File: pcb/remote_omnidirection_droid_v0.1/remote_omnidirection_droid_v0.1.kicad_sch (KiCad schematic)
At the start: 30 parts, among them J1 USB_C_Receptacle_USB2.0, J4 Conn_01x02, Q1 BC846BS, SW1 SW_SPST, U1 USBLC6-2SC6, U3 AZ1117-3.3, U4 AZ1117-5.0, U5 ESP32-S3-WROOM-2-N32R8V

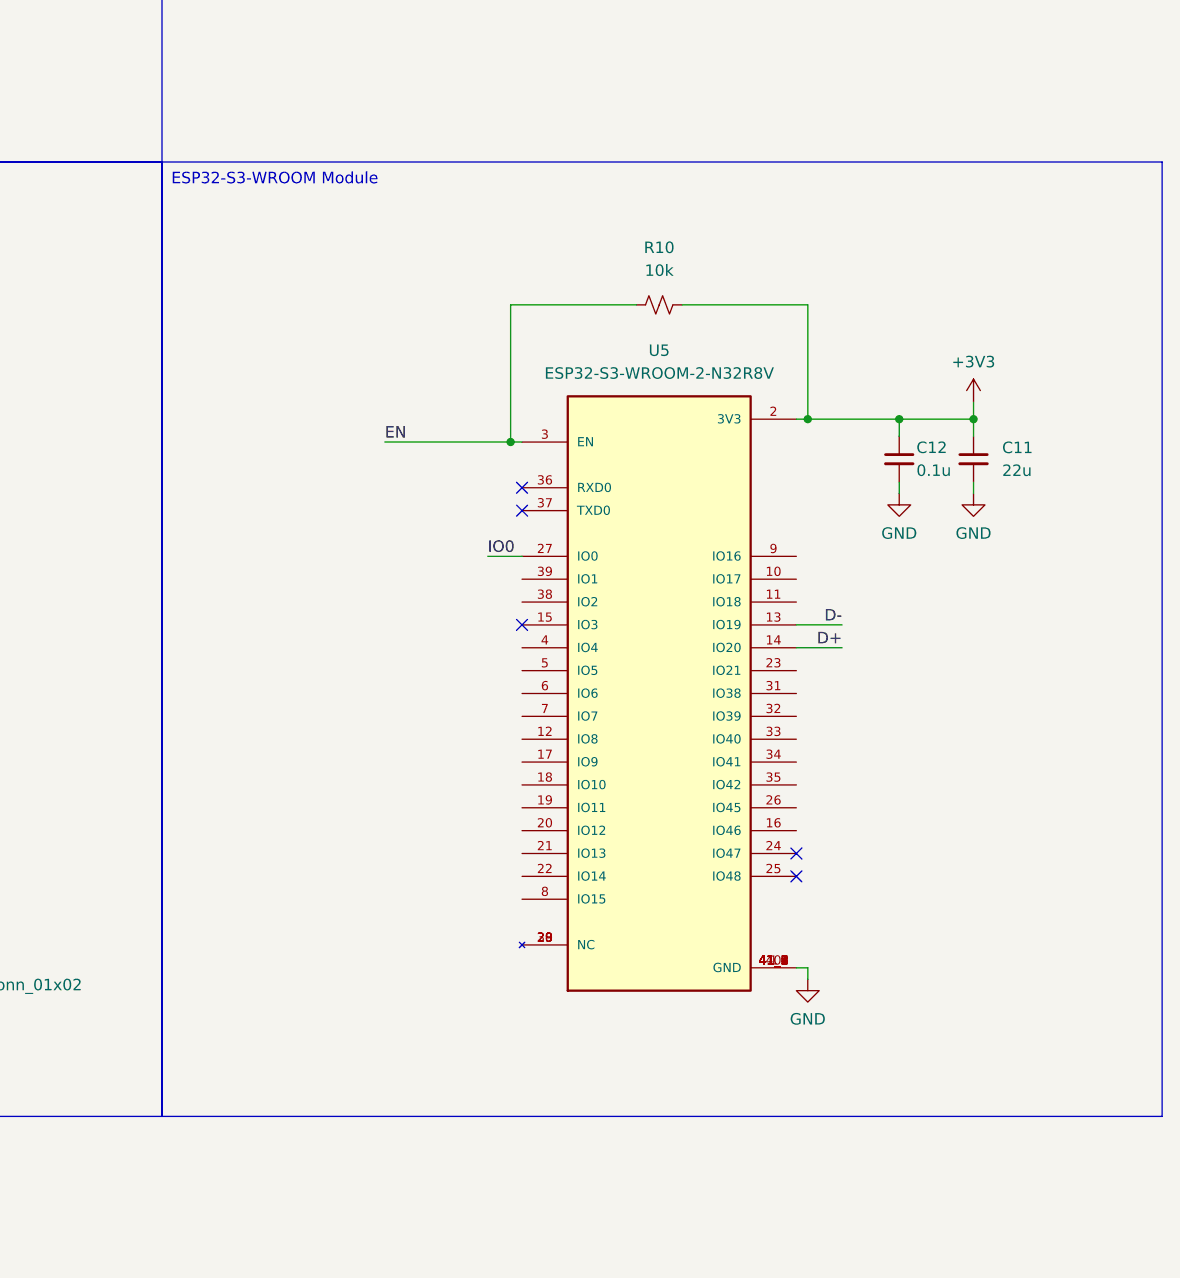
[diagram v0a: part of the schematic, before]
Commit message: poorly designed a PCB
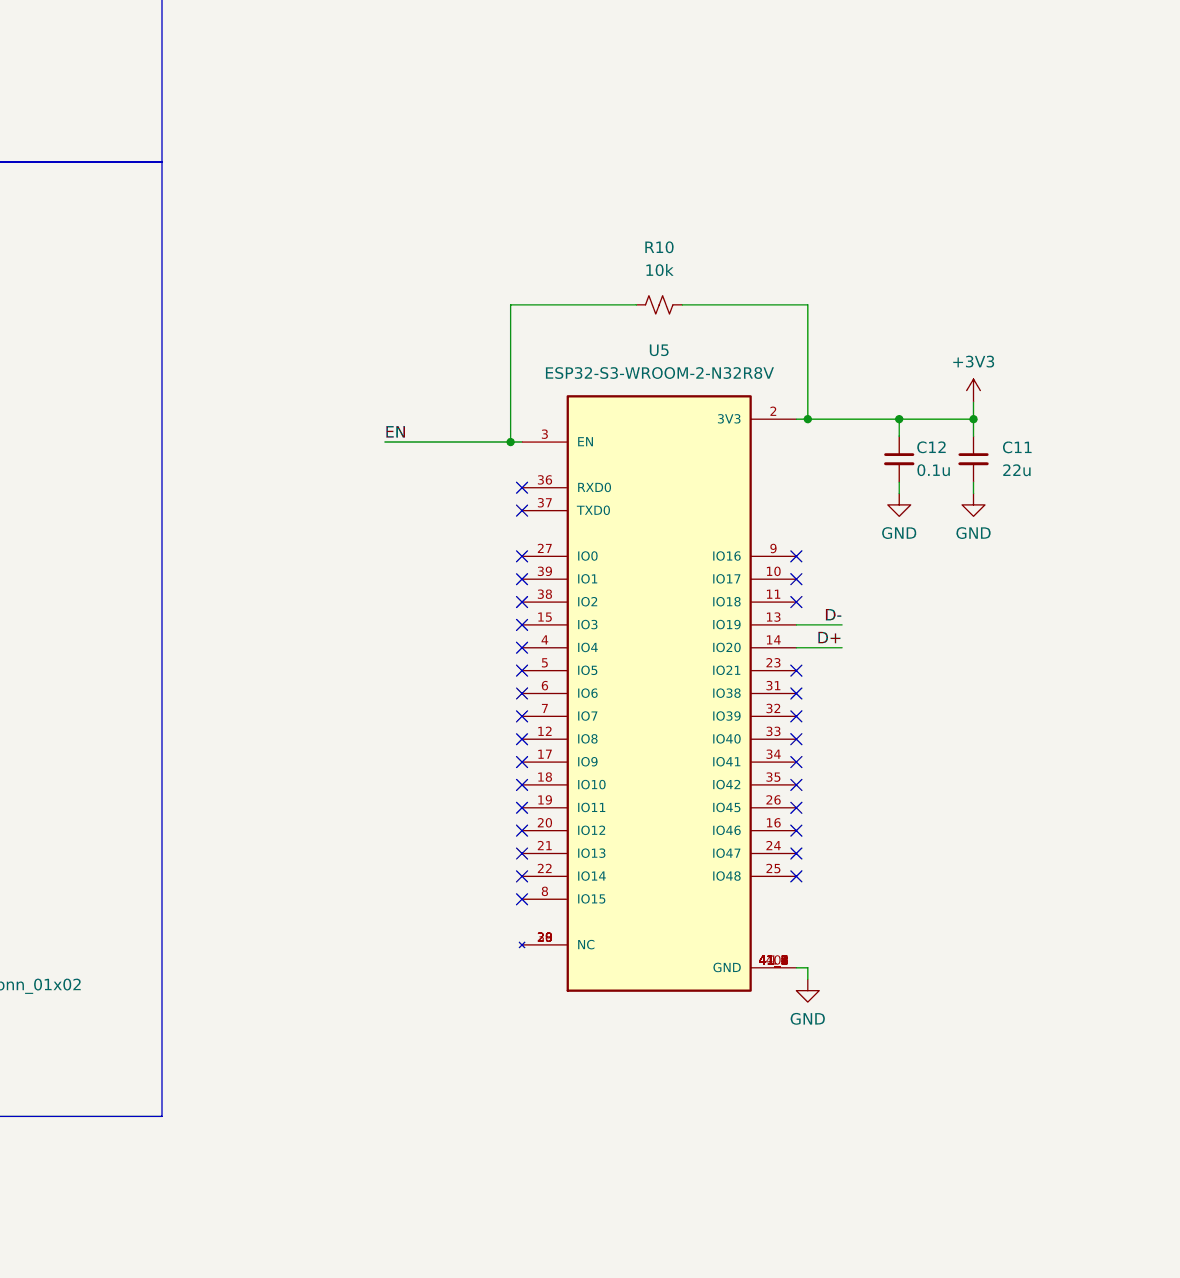
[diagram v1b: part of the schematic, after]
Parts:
- C11, C12, C17: footprint (none) -> Capacitor_SMD:C_1206_3216Metric_Pad1.33x1.80mm_HandSolder
- D1, D2, D8, D9: footprint (none) -> LED_SMD:LED_1206_3216Metric_Pad1.42x1.75mm_HandSolder
- D3, D7: footprint (none) -> Diode_SMD:D_1206_3216Metric_Pad1.42x1.75mm_HandSolder
- J4: footprint (none) -> TestPoint:TestPoint_2Pads_Pitch5.08mm_Drill1.3mm
- R10, R11, R5, R6, R7, R8: footprint (none) -> Resistor_SMD:R_1206_3216Metric_Pad1.30x1.75mm_HandSolder
- U5: footprint ESP32-S3-WROOM-2-N32R8V:XCVR_ESP32-S3-WROOM-2-N32R8V -> ESP32 S3:XCVR_ESP32-S3-WROOM-2-N32R8V
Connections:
- net IO0: no longer names the net of U5.27 (IO0)
- no-connect marks 7 -> 33
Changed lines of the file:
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@@
   (junction (at 56.515 132.715) (diameter 0) (color 0 0 0 0)
   )
+  (no_connect (at 165.1 160.02))
+  (no_connect (at 195.58 167.64))
+  (no_connect (at 195.58 165.1))
+  (no_connect (at 195.58 157.48))
+  (no_connect (at 165.1 162.56))
+  (no_connect (at 165.1 167.64))
   (no_connect (at 165.1 137.16))
+  (no_connect (at 165.1 147.32))
+  (no_connect (at 195.58 162.56))
+  (no_connect (at 165.1 144.78))
+  (no_connect (at 165.1 180.34))
+  (no_connect (at 195.58 142.24))
+  (no_connect (at 165.1 177.8))
+  (no_connect (at 195.58 170.18))
   (no_connect (at 64.135 75.565))
+  (no_connect (at 195.58 147.32))
   (no_connect (at 195.58 175.26))
+  (no_connect (at 165.1 152.4))
+  (no_connect (at 195.58 144.78))
+  (no_connect (at 165.1 170.18))
   (no_connect (at 195.58 177.8))
   (no_connect (at 165.1 134.62))
+  (no_connect (at 165.1 175.26))
+  (no_connect (at 195.58 160.02))
+  (no_connect (at 195.58 154.94))
+  (no_connect (at 165.1 172.72))
   (no_connect (at 165.1 149.86))
+  (no_connect (at 195.58 172.72))
+  (no_connect (at 165.1 154.94))
+  (no_connect (at 165.1 157.48))
   (no_connect (at 64.135 73.025))
+  (no_connect (at 165.1 142.24))
+  (no_connect (at 165.1 165.1))
   (wire (pts (xy 83.185 187.325) (xy 94.615 187.325))
     (stroke (width 0) (type default))
@@
     (stroke (width 0) (type default))
   )
-  (wire (pts (xy 161.29 142.24) (xy 165.1 142.24))
-    (stroke (width 0) (type default))
-  )
   (wire (pts (xy 31.75 215.9) (xy 38.735 215.9))
     (stroke (width 0) (type default))
@@
     (stroke (width 0) (type default))
   )
-  (text_box "ESP32-S3-WROOM Module"
-    (at 125.095 98.425 0) (size 111.125 106.045)
+  (text_box "Enable/Reset Switch"
+    (at 13.335 204.47 0) (size 45.72 27.305)
     (stroke (width 0) (type default))
     (fill (type none))
     (effects (font (size 1.27 1.27)) (justify left top))
   )
-  (text_box "Enable/Reset Switch"
-    (at 13.335 204.47 0) (size 45.72 27.305)
+  (text_box "Power Management"
+    (at 13.335 98.425 0) (size 111.76 106.045)
     (stroke (width 0) (type default))
     (fill (type none))
     (effects (font (size 1.27 1.27)) (justify left top))
   )
-  (text_box "Power Management"
-    (at 13.335 98.425 0) (size 111.76 106.045)
+  (text_box "USB-C + ESD Protection"
+    (at 13.335 34.29 0) (size 111.76 64.135)
     (stroke (width 0) (type default))
     (fill (type none))
     (effects (font (size 1.27 1.27)) (justify left top))
   )
-  (text_box "USB-C + ESD Protection"
-    (at 13.335 34.29 0) (size 111.76 64.135)
+  (text_box "Power Flags"
+    (at 13.335 13.335 0) (size 111.76 20.955)
     (stroke (width 0) (type default))
     (fill (type none))
     (effects (font (size 1.27 1.27)) (justify left top))
   )
-  (text_box "Power Flags"
-    (at 13.335 13.335 0) (size 111.76 20.955)
-    (stroke (width 0) (type default))
-    (fill (type none))
-    (effects (font (size 1.27 1.27)) (justify left top))
-  )
   (label "LED_BATT" (at 83.185 187.325 0) (fields_autoplaced)
     (effects (font (size 1.27 1.27)) (justify left bottom))
@@
     (effects (font (size 1.27 1.27)) (justify left bottom))
   )
-  (label "IO0" (at 161.29 142.24 0) (fields_autoplaced)
-    (effects (font (size 1.27 1.27)) (justify left bottom))
-  )
   (label "EN" (at 52.705 215.9 180) (fields_autoplaced)
     (effects (font (size 1.27 1.27)) (justify right bottom))
@@
       (effects (font (size 1.27 1.27)))
     )
-    (property "Footprint" "ESP32-S3-WROOM-2-N32R8V:XCVR_ESP32-S3-WROOM-2-N32R8V" (at 180.34 157.48 0)
+    (property "Footprint" "ESP32 S3:XCVR_ESP32-S3-WROOM-2-N32R8V" (at 180.34 157.48 0)
       (effects (font (size 1.27 1.27)) (justify bottom) hide)
     )
@@
       (effects (font (size 1.27 1.27)))
     )
-    (property "Footprint" "" (at 81.915 164.465 0)
+    (property "Footprint" "Resistor_SMD:R_1206_3216Metric_Pad1.30x1.75mm_HandSolder" (at 81.915 164.465 0)
       (effects (font (size 1.27 1.27)) hide)
     )
@@
       (effects (font (size 1.27 1.27)))
     )
-    (property "Footprint" "" (at 93.345 158.115 0)
+    (property "Footprint" "LED_SMD:LED_1206_3216Metric_Pad1.42x1.75mm_HandSolder" (at 93.345 158.115 0)
       (effects (font (size 1.27 1.27)) hide)
     )
@@
       (effects (font (size 1.27 1.27)))
     )
-    (property "Footprint" "" (at 30.48 132.715 0)
+    (property "Footprint" "Diode_SMD:D_1206_3216Metric_Pad1.42x1.75mm_HandSolder" (at 30.48 132.715 0)
       (effects (font (size 1.27 1.27)) hide)
     )
@@
       (effects (font (size 1.27 1.27)))
     )
-    (property "Footprint" "" (at 81.915 151.765 0)
+    (property "Footprint" "Resistor_SMD:R_1206_3216Metric_Pad1.30x1.75mm_HandSolder" (at 81.915 151.765 0)
       (effects (font (size 1.27 1.27)) hide)
     )
@@
       (effects (font (size 1.27 1.27)))
     )
-    (property "Footprint" "" (at 62.23 132.715 0)
+    (property "Footprint" "Diode_SMD:D_1206_3216Metric_Pad1.42x1.75mm_HandSolder" (at 62.23 132.715 0)
       (effects (font (size 1.27 1.27)) hide)
     )
@@
       (effects (font (size 1.27 1.27)))
     )
-    (property "Footprint" "" (at 93.345 145.415 0)
+    (property "Footprint" "LED_SMD:LED_1206_3216Metric_Pad1.42x1.75mm_HandSolder" (at 93.345 145.415 0)
       (effects (font (size 1.27 1.27)) hide)
     )
@@
       (effects (font (size 1.27 1.27)))
     )
-    (property "Footprint" "" (at 180.34 114.3 0)
+    (property "Footprint" "Resistor_SMD:R_1206_3216Metric_Pad1.30x1.75mm_HandSolder" (at 180.34 114.3 0)
       (effects (font (size 1.27 1.27)) hide)
     )
@@
       (effects (font (size 1.27 1.27)) (justify left))
     )
-    (property "Footprint" "" (at 102.235 187.325 0)
+    (property "Footprint" "TestPoint:TestPoint_2Pads_Pitch5.08mm_Drill1.3mm" (at 102.235 187.325 0)
       (effects (font (size 1.27 1.27)) hide)
     )
@@
       (effects (font (size 1.27 1.27)))
     )
-    (property "Footprint" "" (at 81.915 145.415 0)
+    (property "Footprint" "Resistor_SMD:R_1206_3216Metric_Pad1.30x1.75mm_HandSolder" (at 81.915 145.415 0)
       (effects (font (size 1.27 1.27)) hide)
     )
@@
       (effects (font (size 1.27 1.27)) (justify left))
     )
-    (property "Footprint" "" (at 207.01 131.445 0)
+    (property "Footprint" "Capacitor_SMD:C_1206_3216Metric_Pad1.33x1.80mm_HandSolder" (at 207.01 131.445 0)
       (effects (font (size 1.27 1.27)) hide)
     )
@@
       (effects (font (size 1.27 1.27)))
     )
-    (property "Footprint" "" (at 93.345 151.765 0)
+    (property "Footprint" "LED_SMD:LED_1206_3216Metric_Pad1.42x1.75mm_HandSolder" (at 93.345 151.765 0)
       (effects (font (size 1.27 1.27)) hide)
     )
@@
       (effects (font (size 1.27 1.27)) (justify left))
     )
-    (property "Footprint" "" (at 215.265 131.445 0)
+    (property "Footprint" "Capacitor_SMD:C_1206_3216Metric_Pad1.33x1.80mm_HandSolder" (at 215.265 131.445 0)
       (effects (font (size 1.27 1.27)) hide)
     )
@@
       (effects (font (size 1.27 1.27)))
     )
-    (property "Footprint" "" (at 41.91 107.315 0)
+    (property "Footprint" "Resistor_SMD:R_1206_3216Metric_Pad1.30x1.75mm_HandSolder" (at 41.91 107.315 0)
       (effects (font (size 1.27 1.27)) hide)
     )
@@
       (effects (font (size 1.27 1.27)))
     )
-    (property "Footprint" "" (at 93.345 164.465 0)
+    (property "Footprint" "LED_SMD:LED_1206_3216Metric_Pad1.42x1.75mm_HandSolder" (at 93.345 164.465 0)
       (effects (font (size 1.27 1.27)) hide)
     )
@@
       (effects (font (size 1.27 1.27)) (justify left))
     )
-    (property "Footprint" "" (at 39.37 125.095 0)
+    (property "Footprint" "Capacitor_SMD:C_1206_3216Metric_Pad1.33x1.80mm_HandSolder" (at 39.37 125.095 0)
       (effects (font (size 1.27 1.27)) hide)
     )
@@
       (effects (font (size 1.27 1.27)))
     )
-    (property "Footprint" "" (at 81.915 158.115 0)
-      (effects (font (size 1.27 1.27)) hide)
-    )
+    (property "Footprint" "Resistor_SMD:R_1206_3216Metric_Pad1.30x1.75mm_HandSolder" (at 81.915 158.115 0)
+      (effects (font (size 1.27 1.27)) hide)
+    )
